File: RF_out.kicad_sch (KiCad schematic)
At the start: 20 parts, among them U2 AS179-92LF

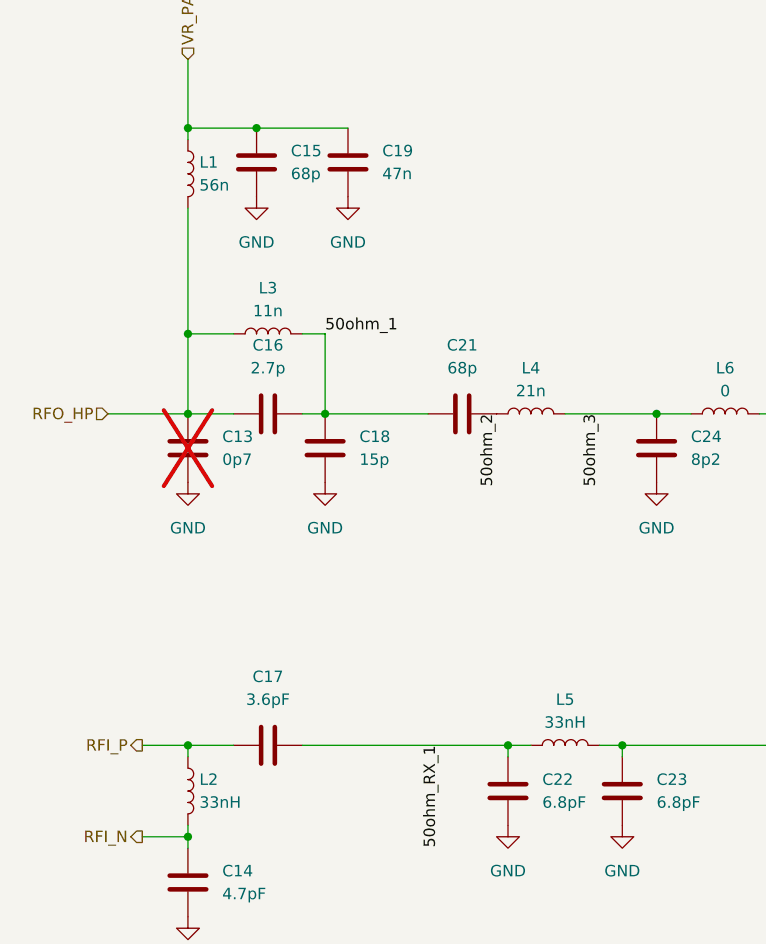
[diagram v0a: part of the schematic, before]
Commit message: Almost ready for production
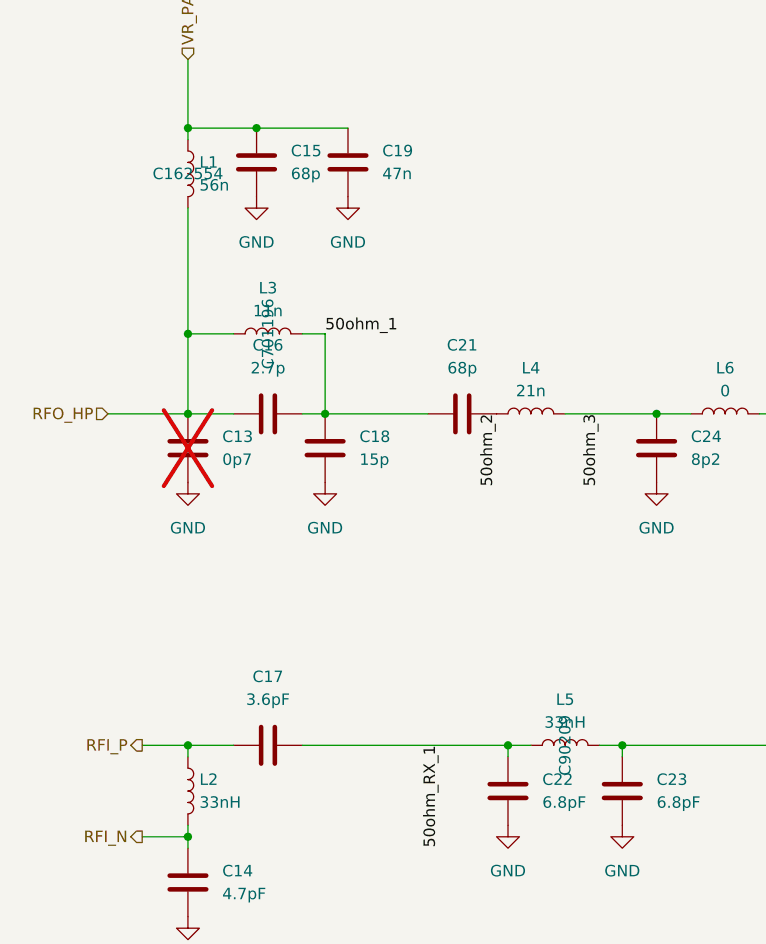
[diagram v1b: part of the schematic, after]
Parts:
- L1: LCSC (none) -> C162554
- L3: LCSC (none) -> C701196
- L5: LCSC (none) -> C90209
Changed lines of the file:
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@@
+			)
+		)
+		(property "LCSC" "C162554"
+			(at 101.6 69.85 0)
+			(effects
+				(font
+					(size 1.27 1.27)
+				)
 			)
 		)
@@
 			)
 		)
+		(property "LCSC" "C701196"
+			(at 110.49 87.63 0)
+			(effects
+				(font
+					(size 1.27 1.27)
+				)
+			)
+		)
 		(pin "2"
 		)
@@
 			)
 		)
+		(property "LCSC" "C90209"
+			(at 143.51 133.35 0)
+			(effects
+				(font
+					(size 1.27 1.27)
+				)
+			)
+		)

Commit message: Fix footprints
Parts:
- L4, L6: footprint Inductor_SMD:L_0402_1005Metric -> Inductor_SMD:L_0603_1608Metric
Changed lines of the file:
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@@
 			)
 		)
-		(property "Footprint" "Inductor_SMD:L_0402_1005Metric"
+		(property "Footprint" "Inductor_SMD:L_0603_1608Metric"
 			(at 139.7 96.52 0)
 			(effects
@@
 			)
 		)
-		(property "Footprint" "Inductor_SMD:L_0402_1005Metric"
+		(property "Footprint" "Inductor_SMD:L_0603_1608Metric"
 			(at 161.29 96.52 0)
 			(effects

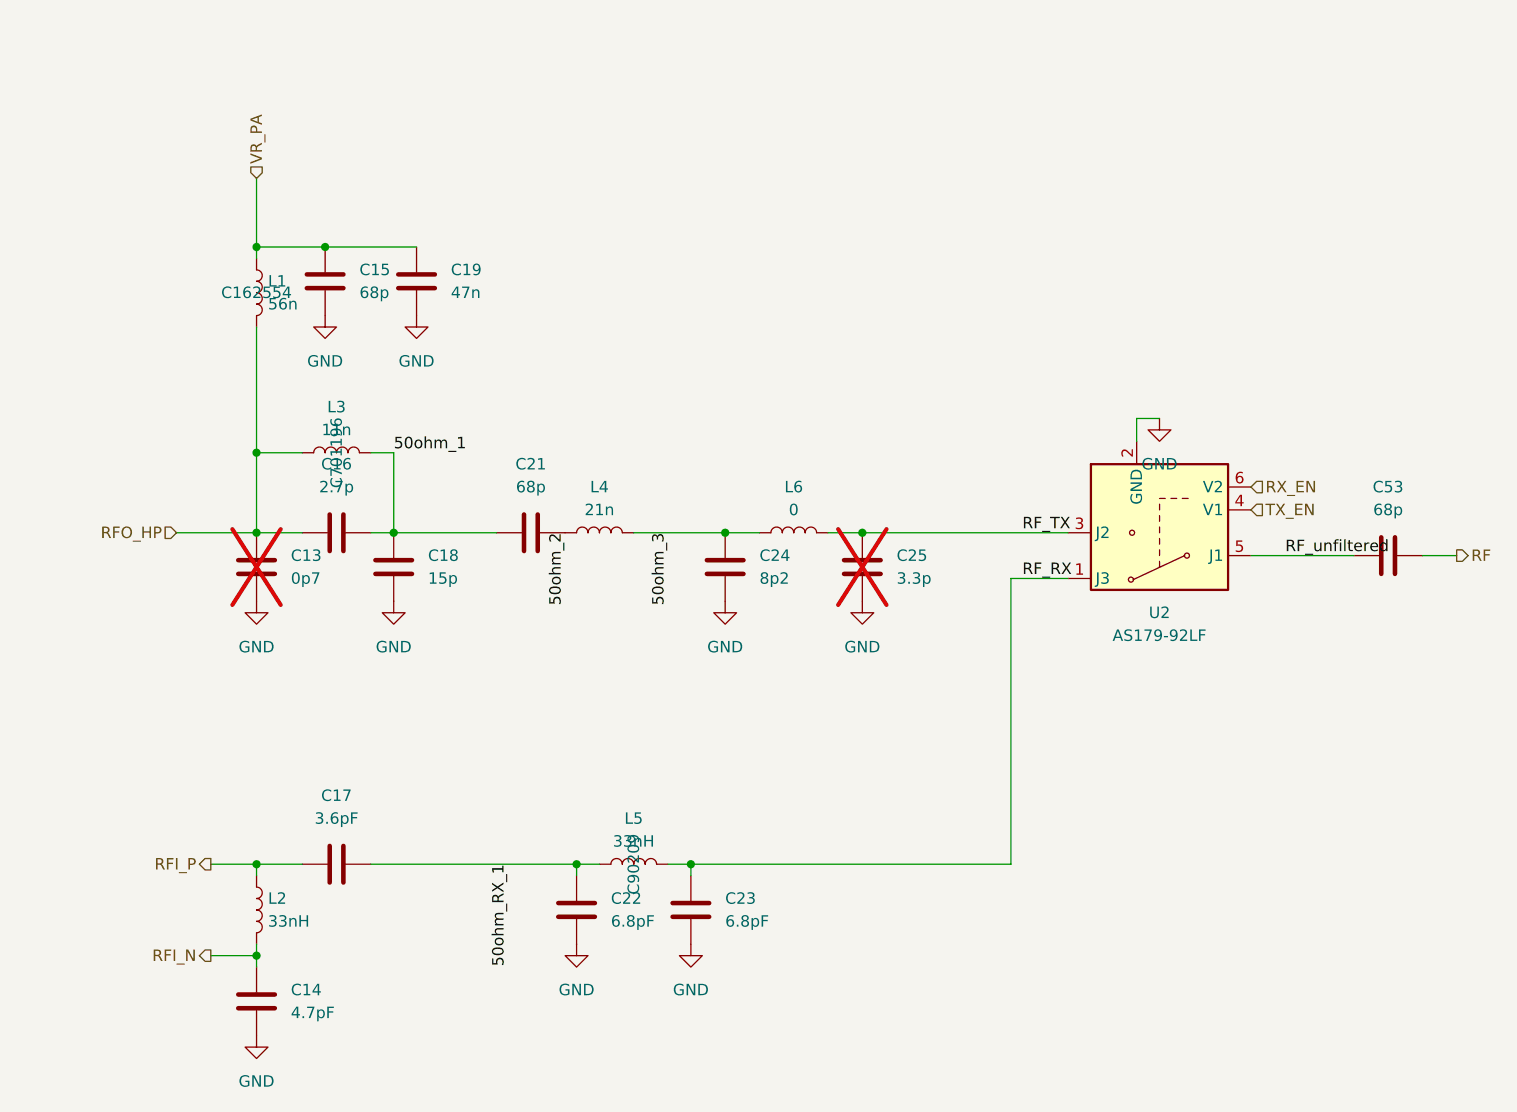
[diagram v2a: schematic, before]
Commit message: Finalize design
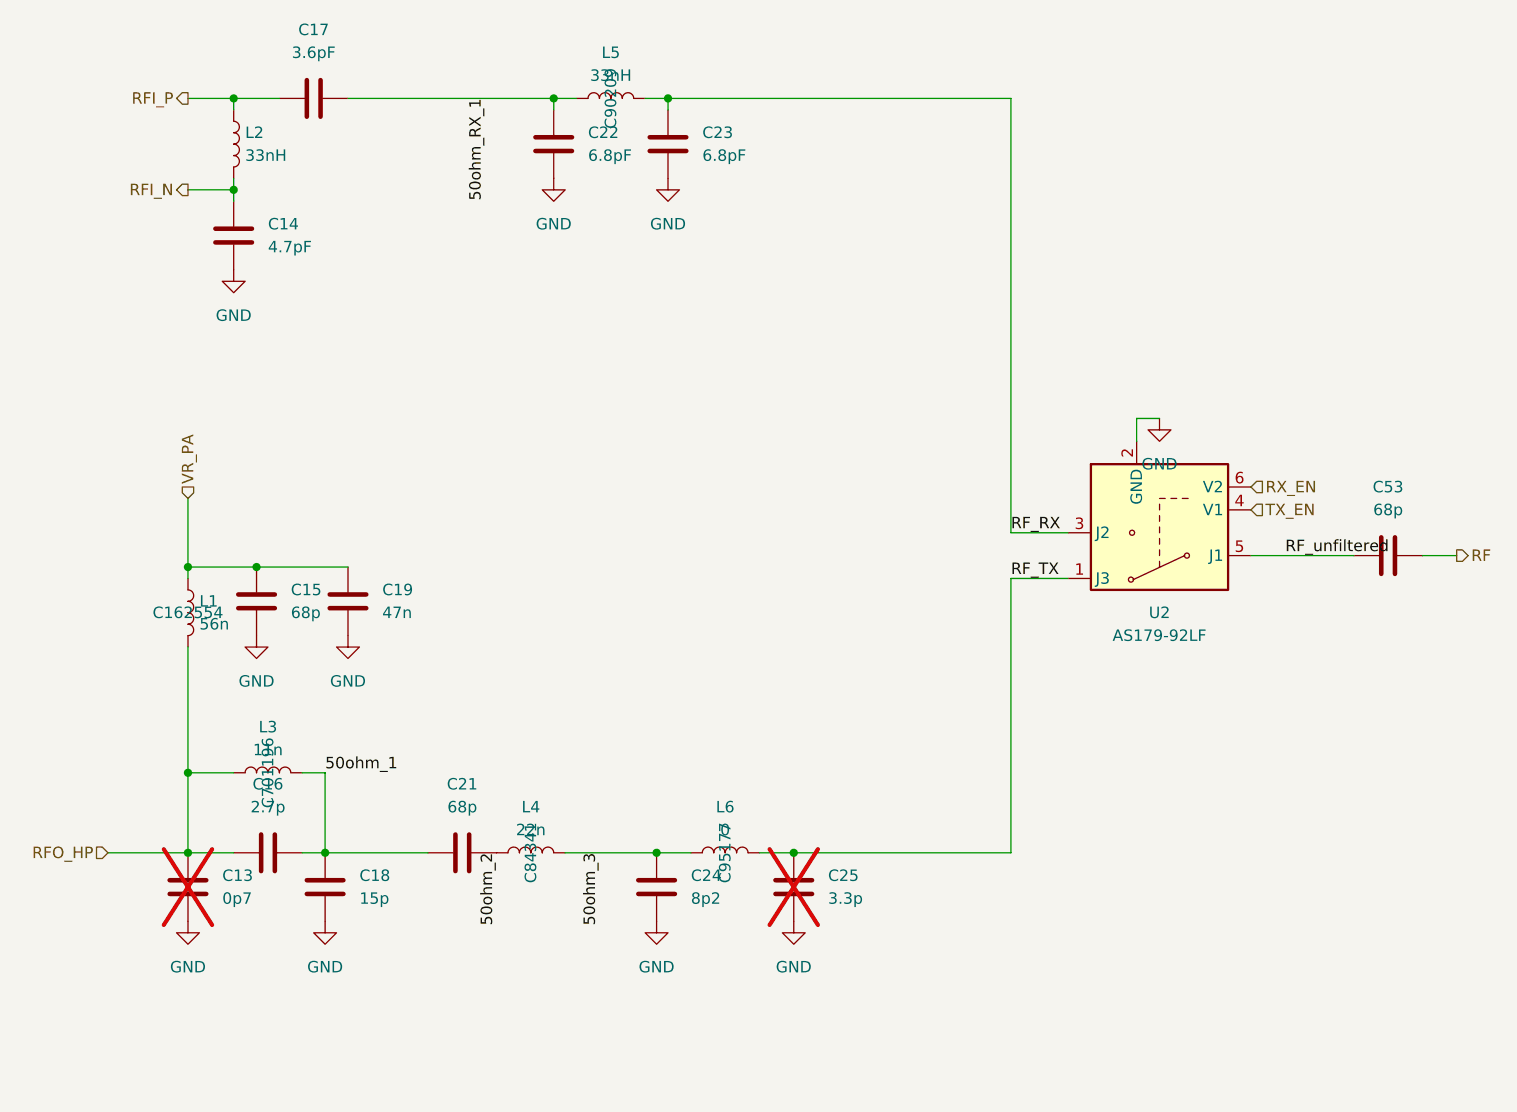
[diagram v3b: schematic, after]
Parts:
- L4: value 21n -> 22n; LCSC (none) -> C84341
- L6: LCSC (none) -> C95177
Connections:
- net RF_RX: now also U2.3 (J2); no longer U2.1 (J3)
- net RF_TX: now also U2.1 (J3); no longer U2.3 (J2)
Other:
- moved on the sheet: C13, C14, C15, C16, C17, C18, C19, C21, C22, C23, C24, C25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
